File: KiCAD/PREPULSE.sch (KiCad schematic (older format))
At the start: 95 parts

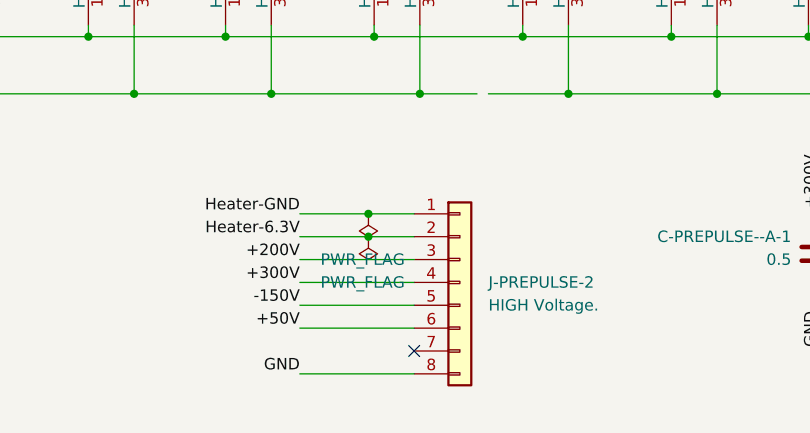
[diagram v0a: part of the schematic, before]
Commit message: Add scfollws.sch
Signed-off-by: John Bradley <flypie@rocketmail.com>
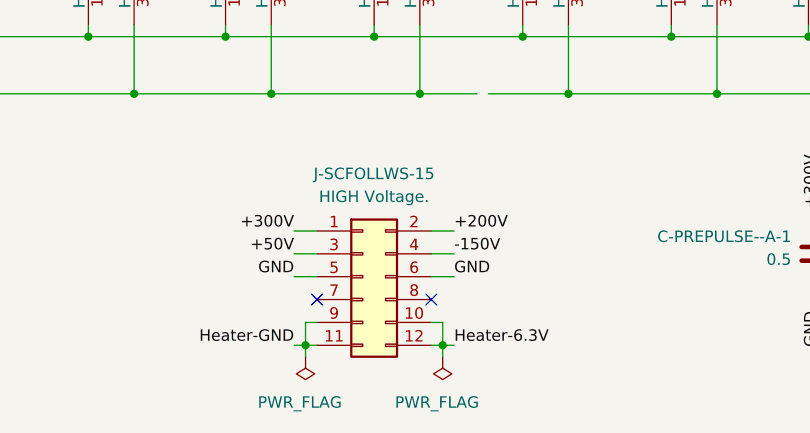
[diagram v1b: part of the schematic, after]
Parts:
- removed J-PREPULSE-2: HIGH Voltage., Connector_TE-Connectivity:TE_MATE-N-LOK_1-770970-x_2x04_P4.14mm_Horizontal, symbol Connector_Generic:Conn_01x08
- added J-SCFOLLWS-15: HIGH Voltage., Connector_TE-Connectivity:TE_MATE-N-LOK_1-770972-x_2x06_P4.14mm_Horizontal, symbol Connector_Generic:Conn_02x06_Odd_Even
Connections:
- net +200V: now also J-SCFOLLWS-15.2 (Pin_2)
- net +300V: now also J-SCFOLLWS-15.1 (Pin_1)
- net +50V: now also J-SCFOLLWS-15.3 (Pin_3)
- net -150V: now also J-SCFOLLWS-15.4 (Pin_4)
- net GND: now also J-SCFOLLWS-15.5 (Pin_5), J-SCFOLLWS-15.6 (Pin_6)
- net Heater-6.3V: now also J-SCFOLLWS-15.10 (Pin_10), J-SCFOLLWS-15.12 (Pin_12)
- net Heater-GND: now also J-SCFOLLWS-15.11 (Pin_11), J-SCFOLLWS-15.9 (Pin_9)
- no-connect marks 14 -> 15
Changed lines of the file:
@@
 $Descr A3 16535 11693
 encoding utf-8
-Sheet 30 32
+Sheet 30 33
 Title "Instruction Gate & Y Shift Position 4.1"
 Date "2020-10-08"
@@
 	1350 10850 1350 11150
 Connection ~ 1350 11150
-Wire Wire Line
-	6925 10425 6725 10425
-Wire Wire Line
-	6925 10325 6725 10325
-$Comp
-L power:PWR_FLAG #FLG0156
-U 1 1 60773F6E
-P 6725 10425
-F 0 "#FLG0156" H 6725 10500 50  0001 C CNN
-F 1 "PWR_FLAG" H 6750 10625 50  0000 C CNN
-F 2 "" H 6725 10425 50  0001 C CNN
-F 3 "~" H 6725 10425 50  0001 C CNN
-	1    6725 10425
-	-1   0    0    1
-$EndComp
-$Comp
-L power:PWR_FLAG #FLG0157
-U 1 1 631D14DD
-P 6725 10325
-F 0 "#FLG0157" H 6725 10400 50  0001 C CNN
-F 1 "PWR_FLAG" H 6750 10525 50  0000 C CNN
-F 2 "" H 6725 10325 50  0001 C CNN
-F 3 "~" H 6725 10325 50  0001 C CNN
-	1    6725 10325
-	-1   0    0    1
-$EndComp
-Connection ~ 6725 10325
-Wire Wire Line
-	6725 10325 6425 10325
-Wire Wire Line
-	6925 10525 6425 10525
-Wire Wire Line
-	6925 10625 6425 10625
-Wire Wire Line
-	6925 10825 6425 10825
-$Comp
-L Connector_Generic:Conn_01x08 J-PREPULSE-2
-U 1 1 60773F7A
-P 7125 10625
-F 0 "J-PREPULSE-2" H 7250 10625 50  0000 L CNN
-F 1 "HIGH Voltage." H 7250 10525 50  0000 L CNN
-F 2 "Connector_TE-Connectivity:TE_MATE-N-LOK_1-770970-x_2x04_P4.14mm_Horizontal" H 7125 10625 50  0001 C CNN
-F 3 "~" H 7125 10625 50  0001 C CNN
-	1    7125 10625
-	1    0    0    -1
-$EndComp
-Connection ~ 6725 10425
-Wire Wire Line
-	6725 10425 6425 10425
-NoConn ~ 6925 10925
-Text Label 6425 10325 2    50   ~ 0
-Heater-GND
-Text Label 6425 10425 2    50   ~ 0
-Heater-6.3V
-Text Label 6425 10525 2    50   ~ 0
-+200V
-Text Label 6425 10625 2    50   ~ 0
-+300V
-Text Label 6425 10725 2    50   ~ 0
--150V
-Text Label 6425 10825 2    50   ~ 0
-+50V
 Text Label 1000 10900 2    50   ~ 0
 Heater-6.3V
 Text Label 1000 11150 2    50   ~ 0
 Heater-GND
-Text Label 6425 11025 2    50   ~ 0
-GND
-Wire Wire Line
-	6425 11025 6925 11025
 $Comp
 L Device:C C-PREPULSE-6
-U 1 1 60773F75
+U 1 1 60A71AAC
 P 11400 10500
 F 0 "C-PREPULSE-6" H 11550 10550 50  0000 L CNN
@@
 $Comp
 L Device:C C-PREPULSE--A-1
-U 1 1 60773F4D
+U 1 1 60A71AA6
 P 8700 10500
 F 0 "C-PREPULSE--A-1" H 8575 10575 50  0000 R CNN
@@
 $Comp
 L Device:C C-PREPULSE-3
-U 1 1 60773F67
+U 1 1 60A71AA9
 P 9550 10500
 F 0 "C-PREPULSE-3" H 9400 10550 50  0000 R CNN
@@
 $Comp
 L NEWValves:EA50 D-PREPULSE-2
-U 2 1 60773F56
+U 2 1 60A71AA8
 P 1900 9050
 F 0 "D-PREPULSE-2" H 1900 9350 50  0000 C CNN
@@
 $Comp
 L NEWValves:EA50 D-PREPULSE-1
-U 2 1 60773F50
+U 2 1 60A71AA7
 P 1250 9050
 F 0 "D-PREPULSE-1" H 1275 9350 50  0000 C CNN
@@
 $Comp
 L NEWValves:VR91 V-PREPULSE-3
-U 2 1 60773F49
+U 2 1 60A71AA5
 P 2550 10500
 F 0 "V-PREPULSE-3" H 2575 11075 50  0000 C CNN
@@
 $Comp
 L NEWValves:VR91 V-PREPULSE-2
-U 2 1 60773F47
+U 2 1 60A71AA4
 P 1900 10500
 F 0 "V-PREPULSE-2" H 1900 11075 50  0000 C CNN
@@
 Text Label 10450 10750 3    50   ~ 0
 GND
-Wire Wire Line
-	6425 10725 6925 10725
 Text Label 8700 10300 1    50   ~ 0
 +300V
@@
 $Comp
 L NEWValves:EA50 D-PREPULSE-1
-U 1 1 631D14DE
+U 1 1 60A71AB1
 P 1600 3400
 F 0 "D-PREPULSE-1" V 1200 3300 50  0000 C CNN
@@
 $Comp
 L Device:R R-PREPULSE-11
-U 1 1 5FAF816B
+U 1 1 60A71A9E
 P 3100 2050
 F 0 "R-PREPULSE-11" V 3350 2050 50  0000 C CNN
@@
 Wire Wire Line
 	6950 9800 7200 9800
+$Comp
+L power:PWR_FLAG #FLG?
+U 1 1 60ABB846
+P 7050 10950
+AR Path="/5F868E46/60ABB846" Ref="#FLG?"  Part="1"
+AR Path="/5F83BB04/60ABB846" Ref="#FLG0156"  Part="1"
+F 0 "#FLG0156" H 7050 11025 50  0001 C CNN
+F 1 "PWR_FLAG" H 7075 11150 50  0000 C CNN
+F 2 "" H 7050 10950 50  0001 C CNN
+F 3 "~" H 7050 10950 50  0001 C CNN
+	1    7050 10950
+	-1   0    0    1
+$EndComp
+$Comp
+L Connector_Generic:Conn_02x06_Odd_Even J-SCFOLLWS-?
+U 1 1 60ABB84C
+P 6700 10600
+AR Path="/5F868E46/60ABB84C" Ref="J-SCFOLLWS-?"  Part="1"
+AR Path="/5F83BB04/60ABB84C" Ref="J-SCFOLLWS-15"  Part="1"
+F 0 "J-SCFOLLWS-15" H 6750 11050 50  0000 C CNN
+F 1 "HIGH Voltage." H 6750 10950 50  0000 C CNN
+F 2 "Connector_TE-Connectivity:TE_MATE-N-LOK_1-770972-x_2x06_P4.14mm_Horizontal" H 6700 10600 50  0001 C CNN
+F 3 "~" H 6700 10600 50  0001 C CNN
+	1    6700 10600
+	1    0    0    -1
+$EndComp
+Text Label 6400 10400 2    50   ~ 0
++300V
+Text Label 7100 10500 0    50   ~ 0
+-150V
+Text Label 6400 10500 2    50   ~ 0
++50V
+Text Label 6400 10600 2    50   ~ 0
+GND
+NoConn ~ 6500 10700
+$Comp
+L power:PWR_FLAG #FLG?
+U 1 1 60ABB857
+P 6450 10950
+AR Path="/5F868E46/60ABB857" Ref="#FLG?"  Part="1"
+AR Path="/5F83BB04/60ABB857" Ref="#FLG0157"  Part="1"
+F 0 "#FLG0157" H 6450 11025 50  0001 C CNN
+F 1 "PWR_FLAG" H 6475 11150 50  0000 C CNN
+F 2 "" H 6450 10950 50  0001 C CNN
+F 3 "~" H 6450 10950 50  0001 C CNN
+	1    6450 10950
+	-1   0    0    1
+$EndComp
+Wire Wire Line
+	6500 10900 6450 10900
+Wire Wire Line
+	6450 10950 6450 10900
+Connection ~ 6450 10900
+Wire Wire Line
+	6450 10900 6400 10900
+Wire Wire Line
+	7000 10900 7050 10900
+Text Label 7100 10900 0    50   ~ 0
+Heater-6.3V
+Connection ~ 7050 10900
+Wire Wire Line
+	7050 10900 7100 10900
+Wire Wire Line
+	7100 10400 7000 10400
+Wire Wire Line
+	7100 10500 7000 10500
+Wire Wire Line
+	7100 10600 7000 10600
+Wire Wire Line
+	6500 10400 6400 10400
+Wire Wire Line
+	6500 10500 6400 10500
+Wire Wire Line
+	6500 10600 6400 10600
+Wire Wire Line
+	6450 10900 6450 10800
+Wire Wire Line
+	6450 10800 6500 10800
+Wire Wire Line
+	7050 10900 7050 10800
+Wire Wire Line
+	7050 10800 7000 10800
+Wire Wire Line
+	7050 10950 7050 10900
+Text Label 7100 10400 0    50   ~ 0
++200V
+Text Label 7100 10600 0    50   ~ 0
+GND
+NoConn ~ 7000 10700
+Text Label 6400 10900 2    50   ~ 0
+Heater-GND
 $EndSCHEMATC
